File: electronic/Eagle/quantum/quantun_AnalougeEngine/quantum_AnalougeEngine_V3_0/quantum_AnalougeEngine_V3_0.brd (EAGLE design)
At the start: 210 x 70 mm, 258 parts, among them IC1 OP275, IC2 OP275, IC3 OP275, IC4 OP275, IC6 OP275, IC8 OP275, IC9 TL072, K5 RELAY_EE2-5NU, K6 RELAY_EE2-5NU, K7 RELAY_EE2-5NU, K8 RELAY_EE2-5NU, Q1 BLM21, U1 ATMEGA2560-16AU, U10 ATMEGA328P-AU, U10_PROG 6PIN_HEADER_SMD_OPEN, U11 ATMEGA328P-AU, U11_PROG 6PIN_HEADER_SMD_OPEN, U12 ULN2003, U1_PROG MAIN_µC, U4 THAT1240, U5 ATMEGA16U2-AU, U5_PROG 6PIN_HEADER_SMD_OPEN, U6 THAT1240, U7 THAT1240, U8 THAT1240

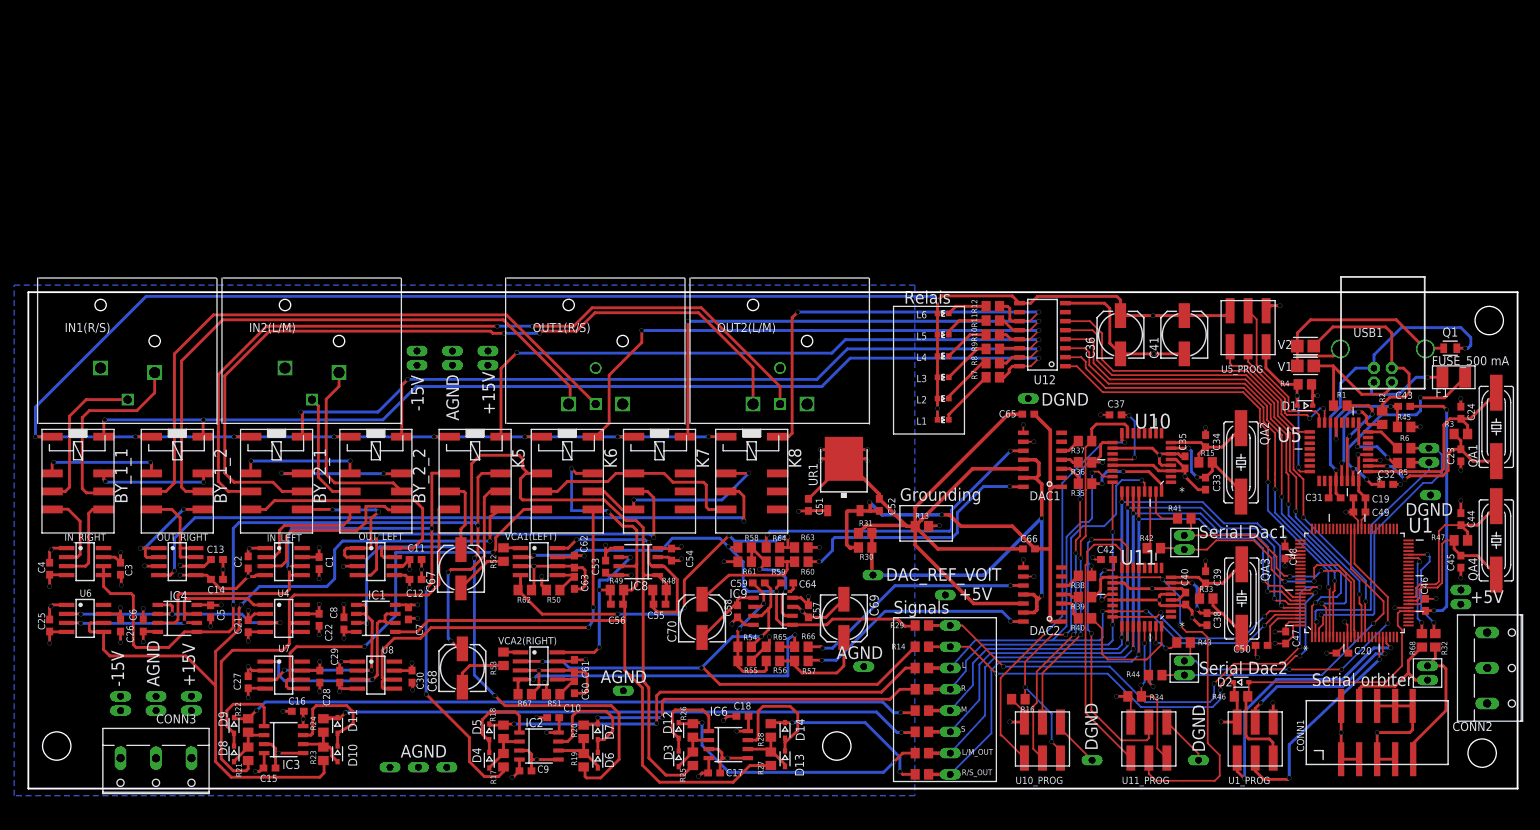
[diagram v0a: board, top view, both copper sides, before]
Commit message: minor changes
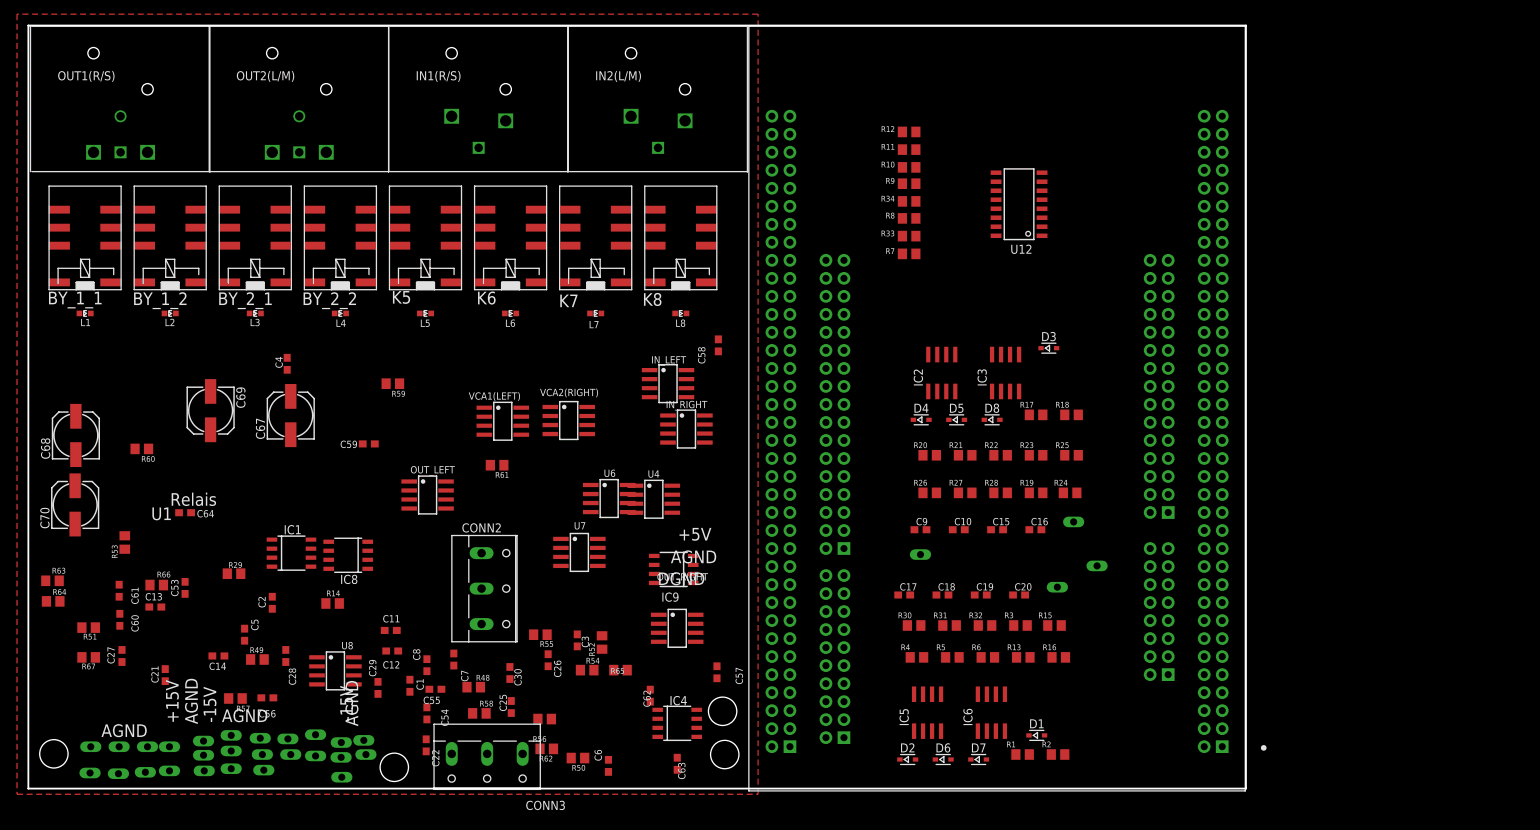
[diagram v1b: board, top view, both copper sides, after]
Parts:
- removed C23, C24, C33, C34, C38, C39, C44, C45, C46: 22pF, C_Sager_Bibliothek:C0603
- removed C31, C35, C40, C51: 1uF, C_Sager_Bibliothek:C0603
- removed C32, C37, C42, C43, C47, C48, C49, C50, C52, C65, C66: 100nF, C_Sager_Bibliothek:C0603
- removed C36, C41: 4,7uF/16V, C_Sager_Bibliothek:153CLV-0605
- removed CONN1: 10PIN_HEADER_SMD, C_Sager_Bibliothek:87832-10
- removed D10, D11, D12, D13, D14, D9: 4148, C_Sager_Bibliothek:SOD323-R
- removed DAC1, DAC2: MCP4922, SPI:SOIC16
- removed F1: FUSE_500 mA, C_Sager_Bibliothek:RESETABLE-FUSE
- removed L, L/M_OUT, M, R, R/S_OUT, S: 0R, C_Sager_Bibliothek:R0805
- removed Q1: BLM21, C_Sager_Bibliothek:RESC2012X85
- removed QA1, QA2, QA3, QA4: 16 MHz, C_Sager_Bibliothek:SM49
- removed R35, R36, R37, R38, R39, R40: 500R, C_Sager_Bibliothek:R0805
- removed R41, R42, R43, R44: 1K, C_Sager_Bibliothek:R0805
- removed R45, R68: 1k, C_Sager_Bibliothek:R0805
- removed R46, R47: 1M, C_Sager_Bibliothek:R0805
- removed TP05, TP06, TP27, TP28, TP29, TP30, TP31, TP32, TP33, TP34, TP35: TPTHT, C_Sager_Bibliothek:THT_PIN
- removed U10, U11: ATMEGA328P-AU, C_Sager_Bibliothek:QFP80P900X900X120-32N
- removed U10_PROG, U11_PROG, U5_PROG: 6PIN_HEADER_SMD_OPEN, C_Sager_Bibliothek:6PIN_HEADER_SMD_OPEN
- removed U1_PROG: MAIN_µC, C_Sager_Bibliothek:6PIN_HEADER_SMD_OPEN
- removed U5: ATMEGA16U2-AU, C_Sager_Bibliothek:QFP80P900X900X120-32N
- removed UR1: 78*, C_Sager_Bibliothek:TO252
- removed USB1: (no value), C_Sager_Bibliothek:SMARTPRJ_PN61729
- removed V1, V2: CG0603ML, C_Sager_Bibliothek:VARC2513X70
- added IC5: NE5532D, linear:SO08
- added L7, L8: SMD_LED_0603, C_Sager_Bibliothek:WL-SMCW_0603
- C59, C64: value 22pF -> 100nF
- D1, D2: value Shotky-CD1206 -> 4148
- IC2, IC3, IC6: value OP275 -> NE5532D; device C_Sager_Bibliothek:SOIC8 -> linear:SO08
- R1, R2: value 22R -> 100k
- R13: value 0R -> 100k
- R15, R3: value 1M -> 0R
- R16, R31: value 10k -> 100k
- R19, R24: value 100k -> 0R
- R21, R26: value 100k -> 180k
- R30: value 10k -> 180k
- R32, R6: value 1k -> 100k
- R33: value 1M -> 500R
- R34: value 10k -> 500R
- R4: value 1M -> 100k
- R48, R49: value 10k -> 20k
- R5: value 1k -> 180k
- U1: value ATMEGA2560-16AU -> NUCLEO-F429ZI; device C_Sager_Bibliothek:QFP50P1600X1600X120-100N -> NUCLEO-F429ZI:MODULE_NUCLEO-F429ZI
- moved TP11 178.6 mm to (24.7, 6.70)
- moved TP12 178.6 mm to (24.7, 4.70)
- moved DGND3 157.5 mm to (44.1, 6.49)
- moved DGND4 145.1 mm to (19.9, 5.90)
- moved CONN2 142.2 mm to (65.2, 28.2)
- moved DGND1 125.2 mm to (24.8, 2.50)
- moved L1 121.9 mm to (8.00, 67.0)
- moved D8 116.8 mm to (135.9, 52.0), turned to 0 degrees
- moved IC3 114.2 mm to (137.8, 58.6), turned to 0 degrees
- moved R22 112.7 mm to (137.1, 47.0), turned to 0 degrees
- moved DGND2 110.6 mm to (44.2, 1.60)
- moved R24 110.3 mm to (146.9, 41.7), turned to 0 degrees
- moved L2 109.7 mm to (20.0, 67.0)
- moved R21 109.5 mm to (132.1, 47.0), turned to 0 degrees
- moved R23 109.0 mm to (142.1, 47.0), turned to 0 degrees
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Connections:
- removed net +5V(ANALOG): C52.2, C65.2, C66.2, DAC1.1, DAC2.1, R30.2, UR1.3
- removed net C_D(+): R2.1, USB1.3, V2.1
- removed net C_D(-): R1.1, USB1.2, V1.1
- removed net C_UVCC: F1.1, USB1.1
- removed net D(+): R2.2, U5.29
- removed net D(-): R1.2, U5.30
- removed net DAC_REF_VOLTAGE: DAC1.11, DAC1.13, DAC2.11, DAC2.13, R30.1, R31.2, TP35.P$1
- removed net L/M_OUT_SIGNAL: L/M_OUT.2, TP03.P$1, U1.93, U10.27, U11.27
- removed net MAIN_µC_AREF: C50.1, U1.98
- removed net MAIN_µC_PB1(SCK): U1.20, U1_PROG.3
- removed net MAIN_µC_PB2(MOSI): U1.21, U1_PROG.4
- removed net MAIN_µC_PB3(MISO): U1.22, U1_PROG.1
- removed net MAIN_µC_RESET: C43.1, C46.1, D2.A, R46.1, U1.30, U1_PROG.5
- removed net MAIN_µC_RX0: R5.2, TP31.P$1, U1.2
- removed net MAIN_µC_RX1: R68.2, U1.45
- removed net MAIN_µC_RX2: R41.2, TP27.P$1, U1.12
- removed net MAIN_µC_RX3: R43.2, TP33.P$1, U1.63
- removed net MAIN_µC_TX0: R6.2, TP32.P$1, U1.3
- removed net MAIN_µC_TX1: R32.2, U1.46
- removed net MAIN_µC_TX2: R42.2, TP28.P$1, U1.13
- removed net MAIN_µC_TX3: R44.2, TP34.P$1, U1.64
- removed net MAIN_µC_XTAL1: C44.2, QA4.2, R47.2, U1.34
- removed net MAIN_µC_XTAL2: C45.2, QA4.1, R47.1, U1.33
- removed net M_SIGNAL: M.2, TP05.P$1, U1.95, U10.25, U11.25
- removed net N$50: D11.C, R24.2, S.1
- removed net N$52: D12.A, D3.C, IC6.1
- removed net N$53: D12.C, L/M_OUT.1, R26.2
- removed net N$54: D13.A, IC6.6, R27.2, R28.1
- removed net N$55: D13.C, D14.A, IC6.7
- removed net N$56: D14.C, R/S_OUT.1, R28.2
- removed net N$63: DAC1.4, R36.2
- removed net N$66: DAC1.5, R37.2
- removed net N$67: DAC2.3, R40.2
- removed net N$68: DAC2.4, R39.2
- removed net N$69: DAC2.5, R38.2
- removed net N$74: C43.2, R45.2, U5.13
- removed net R/S_OUT_SIGNAL: R/S_OUT.2, TP04.P$1, U1.92, U10.28, U11.28
- removed net S_SIGNAL: S.2, TP06.P$1, U1.94, U10.26, U11.26
- removed net UCAP: C31.2, U5.27
- removed net USB_µC_MISO: U5.17, U5_PROG.1
- removed net USB_µC_MOSI: U5.16, U5_PROG.4
- removed net USB_µC_RESET: D1.A, R4.1, U5.24, U5_PROG.5
- removed net USB_µC_RX: R6.1, U5.8
- removed net USB_µC_SCK: U5.15, U5_PROG.3
- removed net USB_µC_TX: R5.1, U5.9
- removed net USB_µC_UGND: C31.1, Q1.2, U5.28, USB1.4
- removed net USB_µC_XTAL1: C24.2, QA1.2, R3.2, U5.1
- removed net USB_µC_XTAL2: C23.2, QA1.1, R3.1, U5.2
- removed net UVCC: C32.1, F1.2, U5.31
- removed net VCA1_A6: U10.19
- removed net VCA1_A7: U10.22
- removed net VCA1_AREF: C37.2, U10.20
- removed net VCA1_D10: U10.14
- removed net VCA1_D11(MOSI): R37.1, U10.15, U10_PROG.4
- removed net VCA1_D12(MISO): U10.16, U10_PROG.1
- removed net VCA1_D13(SCK): R36.1, U10.17, U10_PROG.3
- removed net VCA1_D2: R35.1, U10.32
- removed net VCA1_D3: U10.1
- removed net VCA1_D4: U10.2
- removed net VCA1_D5: U10.9
- removed net VCA1_D6: U10.10
- removed net VCA1_D7: U10.11
- removed net VCA1_D8: U10.12
- removed net VCA1_D9: U10.13
- removed net VCA1_RESET: R16.1, U10.29, U10_PROG.5
- removed net VCA1_µC_RX: R42.1, U10.30
- removed net VCA1_µC_TX: R41.1, U10.31
- removed net VCA2_A6: U11.19
- removed net VCA2_A7: U11.22
- removed net VCA2_AREF: C42.2, U11.20
- removed net VCA2_D10: U11.14
- removed net VCA2_D11(MOSI): R38.1, U11.15, U11_PROG.4
- removed net VCA2_D12(MISO): U11.16, U11_PROG.1
- removed net VCA2_D13(SCK): R39.1, U11.17, U11_PROG.3
- removed net VCA2_D2: R40.1, U11.32
- removed net VCA2_D3: U11.1
- removed net VCA2_D4: U11.2
- removed net VCA2_D5: U11.9
- removed net VCA2_D6: U11.10
- removed net VCA2_D7: U11.11
- removed net VCA2_D8: U11.12
- removed net VCA2_D9: U11.13
- removed net VCA2_RESET: R34.1, U11.29, U11_PROG.5
- removed net VCA2_µC_RX: R44.1, U11.30
- removed net VCA2_µC_TX: R43.1, U11.31
- removed net XTAL1_VCA1: C33.2, QA2.2, R15.2, U10.7
- removed net XTAL1_VCA2: C38.2, QA3.2, R33.2, U11.7
- removed net XTAL2_VCA1: C34.2, QA2.1, R15.1, U10.8
- removed net XTAL2_VCA2: C39.2, QA3.1, R33.1, U11.8
- new net N$10: D3.A, R20.1, R22.2
- new net N$3: D4.C, IC2.2, R17.2, R22.1
- new net N$35: IC2.7, R19.1, R23.2
- new net N$37: D8.C, IC3.2, R18.2, R27.1
- new net N$4: D3.C, D4.A, IC2.1
- net +5V: now also L7.2, L8.2; no longer C19.1, C20.1, C35.2, C36.+, C40.2, C41.+, C47.1, C48.1, C49.1, CONN1.1, CONN1.2, CONN1.3, D1.C, D2.C, DAC1.9, DAC2.9, R16.2, R34.2, R4.2, R46.2, U1.10, U1.100, U1.31, U1.61, U1.80, U10.18, U10.4, U10.6, U10_PROG.2, U11.18, U11.4, U11.6, U11_PROG.2, U1_PROG.2, U5.32, U5.4, U5_PROG.2
- net AGND: now also C19.2, C20.2, IC5.3, IC5.5; no longer C51.1, C52.1, C65.1, C66.1, DAC1.12, DAC2.12, R13.2, R31.1, UR1.2
- net DAC1_OUT(A): no longer DAC1.14
- net DAC1_OUT(B): no longer DAC1.10
- net DAC2_OUT(A): no longer DAC2.14
- net DAC2_OUT(B): no longer DAC2.10
- net DGND: no longer C19.2, C20.2, C23.1, C24.1, C32.2, C33.1, C34.1, C35.1, C36.-, C37.1, C38.1, C39.1, C40.1, C41.-, C42.1, C44.1, C45.1, C46.2, C47.2, C48.2, C49.2, C50.2, CONN1.10, CONN1.5, CONN1.6, CONN1.7, CONN1.8, DAC1.8, DAC2.8, R13.1, R45.1, U1.11, U1.32, U1.62, U1.81, U1.99, U10.21, U10.3, U10.5, U10_PROG.6, U11.21, U11.3, U11.5, U11_PROG.6, U1_PROG.6, U5.3, U5_PROG.6
- net L: now also R1.1, R21.1, R5.1
- net L/M_OUT(VCA1_OUT): no longer R25.1
- net L_SIGNAL: now also R19.2, R3.2, TP03.P$1; no longer L.2, U1.97, U10.23, U11.23
- net M: no longer R21.1
- net MAIN_µC_D2: no longer U1.6
- net MAIN_µC_D3: no longer U1.7
- net MAIN_µC_D4: no longer U1.1
- net MAIN_µC_D5: no longer U1.5
- net MAIN_µC_D6: no longer U1.15
- net MAIN_µC_D7: no longer U1.16
- net N$12: now also D1.A, R4.1, R6.2; no longer U1.23
- net N$16: now also L3.1; no longer L2.1
- net N$20: now also IC2.6, R20.2, R21.2, R23.1; no longer D5.C, L.1, R18.2
- net N$26: now also L8.1; no longer L6.1
- net N$29: now also L7.1; no longer L5.1
- net N$30: now also L6.1; no longer L4.1
- net N$32: now also L5.1; no longer L3.1
- net N$34: now also IC5.6, R13.1, R4.2, R5.2; no longer Q1.1, USB1.P$1, USB1.P$2, V1.2, V2.2
- net N$36: now also IC5.7, R13.2, R3.1; no longer DAC1.3, R35.2
- net N$38: now also D5.C, D8.A, IC3.1; no longer D4.A, IC2.2, R17.2, R18.1
- net N$39: now also R25.1, R27.2; no longer D4.C, IC2.1
- net N$40: now also IC3.6, R25.2, R26.2, R28.1; no longer D6.A, IC2.6, R19.2, R20.1
- net N$41: now also IC3.7, R24.1, R28.2; no longer D6.C, D7.A, IC2.7
- net N$42: now also IC6.2, R2.2, R31.1; no longer R.1, R20.2
- net N$44: now also D6.C, D7.A, IC6.1; no longer D8.A, IC3.2, R21.2, R22.1
- net N$46: now also D6.A, R16.1, R31.2; no longer D8.C, D9.A, IC3.1
- net N$47: now also IC6.6, R16.2, R30.2, R32.1; no longer D9.C, M.1, R22.2
- net N$48: now also IC6.7, R15.1, R32.2; no longer D10.A, IC3.6, R23.2, R24.1
- net N$49: now also L2.1, R33.2; no longer D10.C, D11.A, IC3.7
- net N$51: now also L4.1, R34.2; no longer D3.A, IC6.2, R25.2, R26.1
- net N$6: now also D2.C, IC5.2, R1.2, R6.1; no longer CONN1.4, R68.1, TP29.P$1
- net N$9: now also D1.C, D2.A, IC5.1; no longer CONN1.9, R32.1, TP30.P$1
- net OUT1_DRIVER: now also R33.1
- net OUT2_DRIVER: now also R34.1
- net R: now also R18.1, R2.1, R26.1, R30.1; no longer R19.1
- net R/S_OUT(VCA2_OUT): no longer R27.1
- net R_SIGNAL: now also R15.2, R24.2, TP04.P$1; no longer R.2, U1.96, U10.24, U11.24
- net S: no longer R23.1
- net V+: now also C20.1, IC5.8; no longer C51.2, UR1.1
- net V-: now also C19.1, IC5.4
- net VCA1_EC+: no longer U1.90
- net VCA2_EC+: no longer U1.91
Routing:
- net +5V: track 404.9 -> 0.00 mm, vias 25 -> 0
- net AGND: track 264.6 -> 0.00 mm, vias 36 -> 0
- net OUT1_DRIVER: track 147.0 -> 0.00 mm, vias 3 -> 0
- net R: track 147.0 -> 0.00 mm, vias 4 -> 0
- net DGND: track 141.1 -> 0.00 mm, vias 27 -> 0
- net OUT2_DRIVER: track 126.4 -> 0.00 mm, vias 3 -> 0
- net L/M_OUT(VCA1_OUT): track 120.3 -> 0.00 mm, vias 2 -> 0
- net S: track 113.9 -> 0.00 mm, vias 2 -> 0
- net N$17: track 112.5 -> 0.00 mm, vias 2 -> 0
- net R/S_OUT(VCA2_OUT): track 111.1 -> 0.00 mm, vias 2 -> 0
- net N$15: track 110.4 -> 0.00 mm, vias 2 -> 0
- net L: track 107.5 -> 0.00 mm, vias 4 -> 0
- net R/S_OUT_SIGNAL: track 98.8 -> 0.00 mm, vias 3 -> 0
- net N$47: track 97.8 -> 0.00 mm, vias 2 -> 0
- net L/M_OUT_SIGNAL: track 96.9 -> 0.00 mm, vias 3 -> 0
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- added copper zone on layer 1, net AGND
- removed copper zone on layer 15, net +5V
- removed copper zone on layer 2, net AGND
- removed copper zone on layer 2, net DGND
- removed copper zone on layer 15, net V+
- removed copper zone on layer 16, net V-
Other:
- board size 210 x 70 mm -> 171.7 x 107.6 mm
- board text removed: "DAC_REF_VOlT"
- board text removed: "Grounding"
- board text removed: "Serial Dac1"
- board text removed: "Serial Dac2"
- board text removed: "Serial orbiter"
- board text removed: "Signals"
